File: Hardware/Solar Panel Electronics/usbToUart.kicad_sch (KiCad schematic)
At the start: 17 parts, among them J6 USB_C_Receptacle_USB2.0, U5 INTERFACE-CP2102-GMR(QFN28)

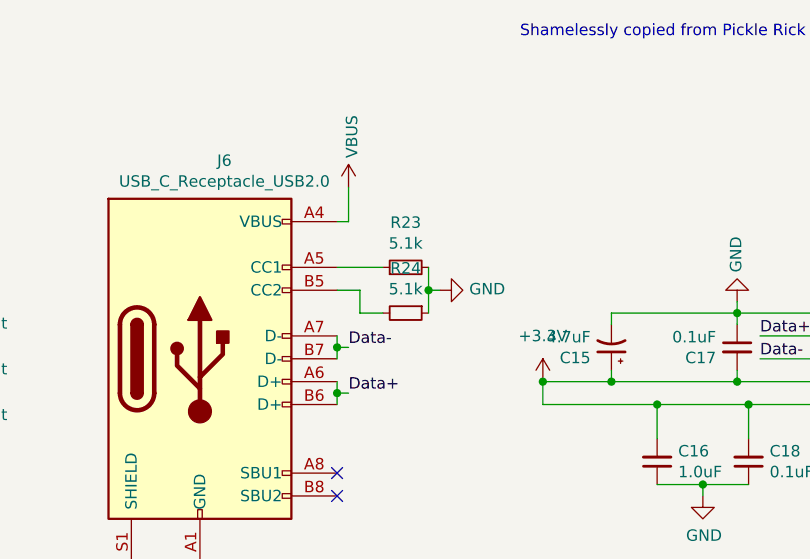
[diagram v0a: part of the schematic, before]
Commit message: ICARUS v2
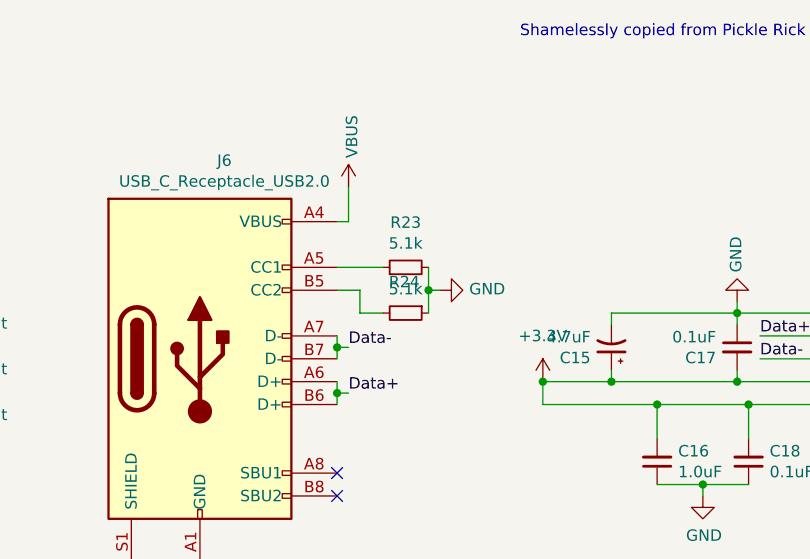
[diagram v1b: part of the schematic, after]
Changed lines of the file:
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@@
   (symbol (lib_id "Device:R_Small") (at 121.92 69.85 270) (unit 1)
     (in_bom yes) (on_board yes)
-    (property "Reference" "R24" (id 0) (at 121.92 64.8716 90))
+    (property "Reference" "R24" (id 0) (at 121.7676 66.3956 90))
     (property "Value" "5.1k" (id 1) (at 121.92 67.183 90))
     (property "Footprint" "Resistor_SMD:R_0603_1608Metric" (id 2) (at 121.92 69.85 0)
